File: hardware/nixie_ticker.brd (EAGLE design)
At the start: 127 x 61 mm, 34 parts

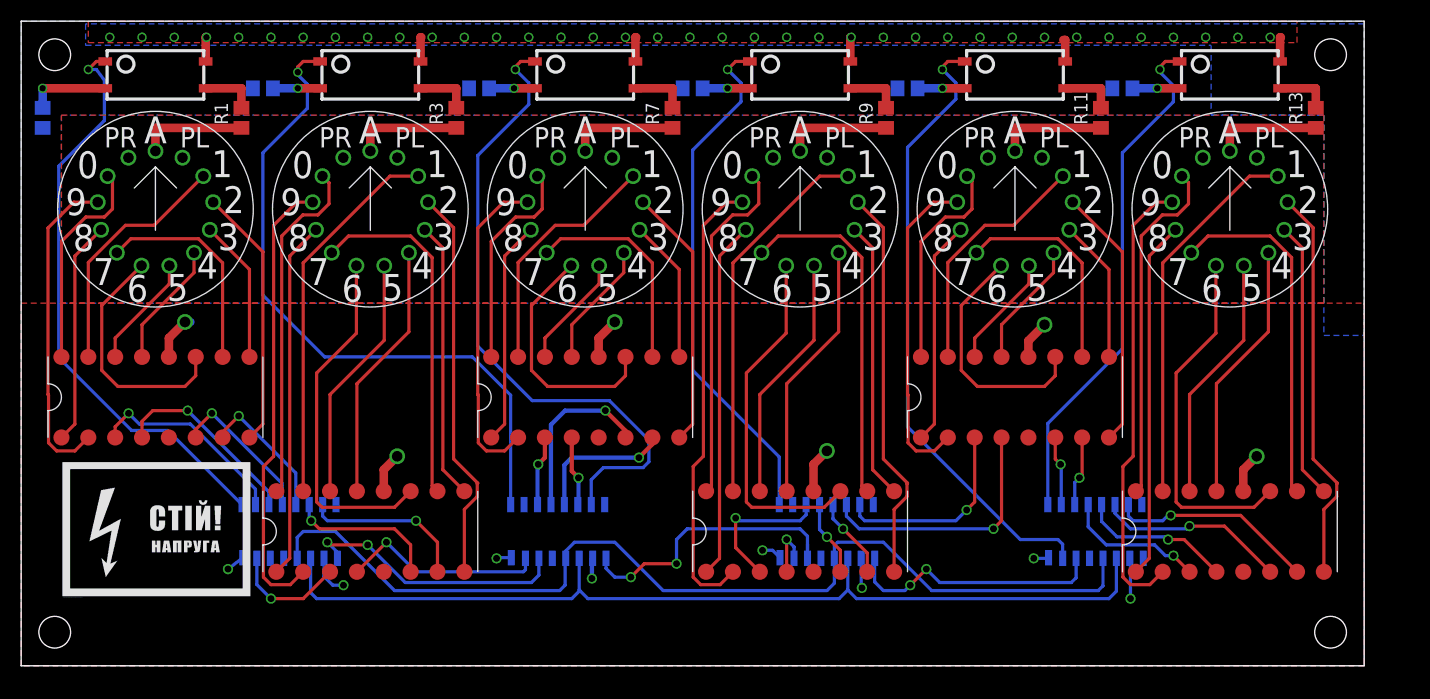
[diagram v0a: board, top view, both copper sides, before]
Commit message: Updates 6-29
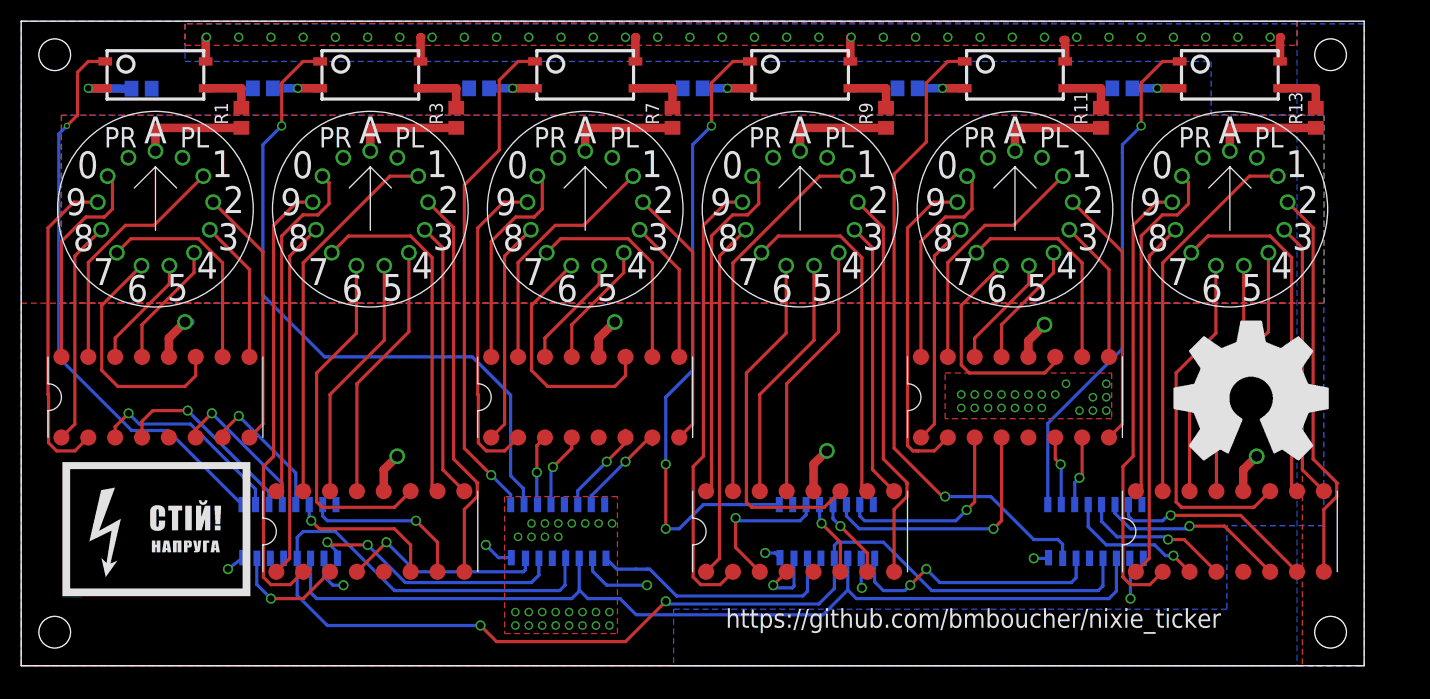
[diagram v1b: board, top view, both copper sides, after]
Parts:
- moved R2 9.76 mm to (11.4, 54.6), turned to 0 degrees
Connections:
- net N$42: now also U$4.P$5; no longer U$4.P$2
- net N$43: now also U$4.P$2; no longer U$4.P$1
- net N$45: now also U$4.P$6; no longer U$4.P$4
- net N$46: now also U$4.P$7; no longer U$4.P$5
- net N$48: now also U$4.P$4; no longer U$4.P$6
- net N$49: now also U$4.P$1; no longer U$4.P$7
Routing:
- net N$86: track 95.6 -> 126.6 mm, vias 0 -> 2
- net N$49: track 61.4 -> 47.4 mm
- net N$56: track 49.4 -> 60.1 mm, vias 1 -> 3
- net N$45: track 16.6 -> 8.85 mm
- net +5V: track 19.0 -> 25.2 mm
- net N$46: track 13.5 -> 9.53 mm
- net N$21: track 27.3 -> 23.8 mm, vias 2 -> 0
- net N$97: track 23.2 -> 21.1 mm
- net N$103: track 7.76 -> 5.69 mm
- net N$60: track 59.4 -> 61.3 mm
- net N$53: track 5.12 -> 6.62 mm
- net N$85: track 49.3 -> 48.0 mm
- net N$87: track 90.4 -> 91.7 mm
- net N$28: track 55.1 -> 53.9 mm
- net N$48: track 6.64 -> 7.17 mm
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- added copper zone on layer 1, net GND
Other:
- board text added: "https://github.com/bmboucher/nixie_ticker"

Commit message: Updates 6-29
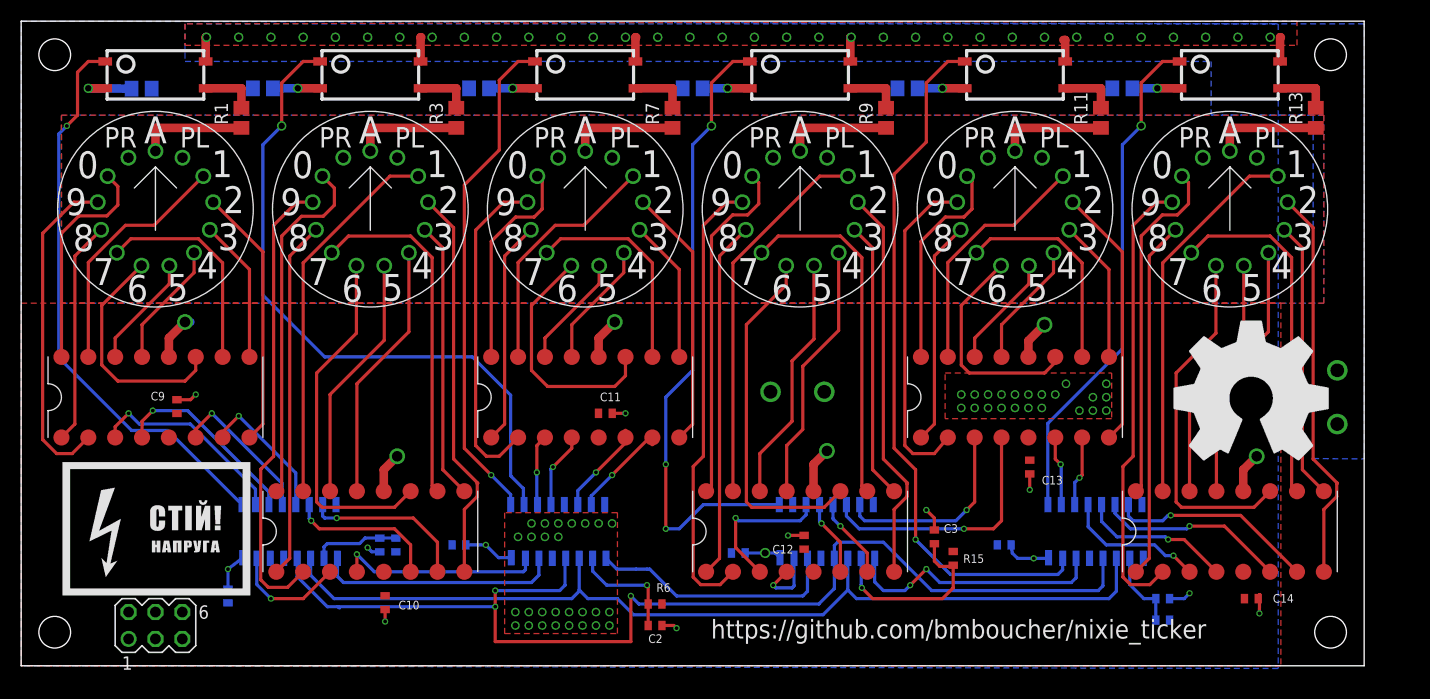
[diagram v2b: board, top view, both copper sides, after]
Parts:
- added C1, C10, C11, C12, C13, C14, C2, C3, C4, C5, C6, C7, C8, C9: (no value), resistor:C0402
- added R15, R16, R5, R6: (no value), resistor:R0402
- added SV1: (no value), con-lstb:MA03-2
- added U$17, U$24: ZKFDS, nixie_ticker:ZKFDS
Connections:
- new net N$108: C2.1, R6.1, U$4.P$10
- new net N$109: C1.1, R5.1, U$3.P$10
- new net N$110: C3.1, R15.1, U$9.P$10
- new net N$111: C8.1, R16.1, U$10.P$10
- new net N$159: SV1.4
- net +5V: now also C10.1, C11.1, C12.1, C13.1, C14.1, C4.1, C5.1, C6.1, C7.1, C9.1, R15.2, R16.2, R5.2, R6.2, SV1.6; no longer U$10.P$10, U$3.P$10, U$4.P$10, U$9.P$10
- net GND: now also C1.2, C10.2, C11.2, C12.2, C13.2, C14.2, C2.2, C3.2, C4.2, C5.2, C6.2, C7.2, C8.2, C9.2, SV1.2, U$24.P$1, U$24.P$2
- net N$86: now also SV1.1
- net N$87: now also SV1.3
- net N$88: now also SV1.5
- net V+: now also U$17.P$1, U$17.P$2
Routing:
- net N$86: track 126.6 -> 108.2 mm, vias 2 -> 3
- net N$110: track 0.00 -> 18.0 mm, vias 0 -> 1
- net GND: track 24.0 -> 37.3 mm, vias 55 -> 63
- net N$108: track 0.00 -> 10.8 mm, vias 0 -> 1
- net N$109: track 0.00 -> 8.22 mm
- net N$111: track 0.00 -> 7.61 mm
- net +5V: track 25.2 -> 19.8 mm, vias 8 -> 6
- net N$60: track 61.3 -> 66.3 mm
- net N$22: track 25.4 -> 22.9 mm, vias 2 -> 0
- net N$7: track 23.2 -> 22.2 mm
- net N$87: track 91.7 -> 90.7 mm
- net N$1: track 20.3 -> 21.3 mm
- net N$40: track 30.7 -> 31.5 mm
- net N$11: track 32.9 -> 33.7 mm
- net N$10: track 30.7 -> 31.4 mm
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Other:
- board text removed: "C:/Users/bmbou/Desktop/Stop_high_voltage_ukrainian_sign.bmp"
